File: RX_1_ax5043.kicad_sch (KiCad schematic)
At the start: 16 parts, among them U201 RFShield_OnePiece, U205 AX5043, U207 TPS22929D

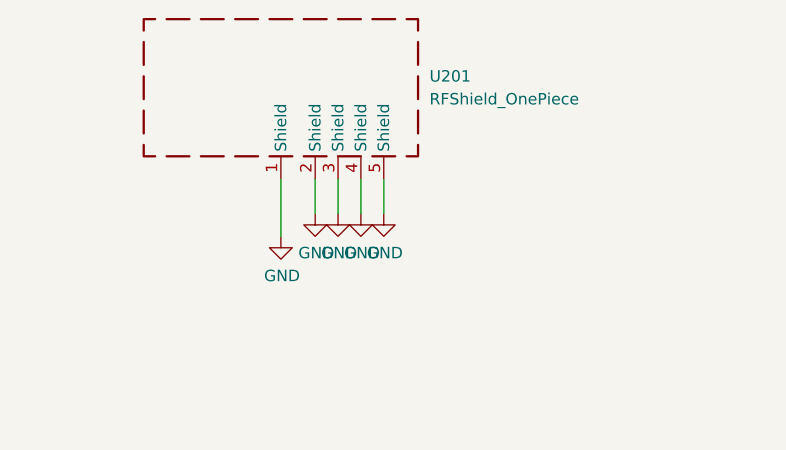
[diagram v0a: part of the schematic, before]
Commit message: More hacking on things
Signed-off-by: Corey Minyard <corey@minyard.net>
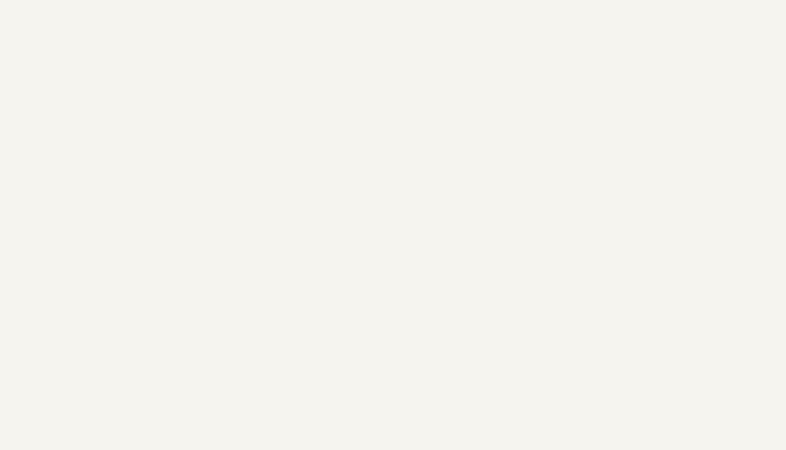
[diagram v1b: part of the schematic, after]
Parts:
- removed U201: RFShield_OnePiece, PacSatDev_misc:RF_SHIELD_BMI_S_201_F_U201, symbol PACSAT_DEV_misc:RF_SHIELD_BOX
